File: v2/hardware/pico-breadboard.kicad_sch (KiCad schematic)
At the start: 39 parts, among them J1 Conn_01x05, J10 MPU6050 CONNECTOR, J11 Conn_01x03, J12 Conn_01x03, J2 LED, J3 5V CONNECTOR, J4 GND CONNECTOR, J5 3.3V CONNECTOR, J6 Conn_01x12, J7 Conn_01x11, J8 SCREEN CONNECTOR, J9 Conn_01x03, Q1 BC817, SW1 SW_SPST, SW2 SW_SPST, SW3 SW_SPST, SW4 SW_SPST, SW5 RotaryEncoder_Switch_MP, U1 Pico

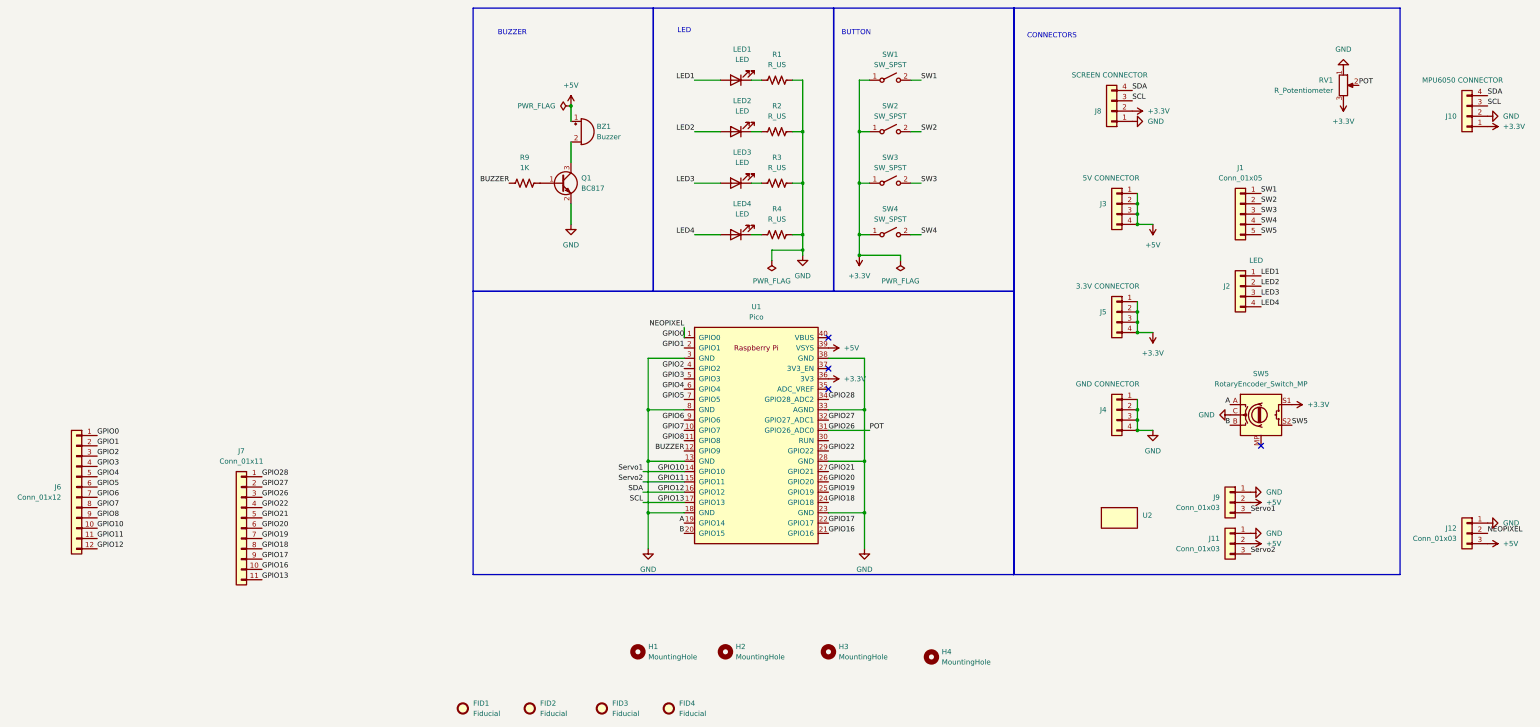
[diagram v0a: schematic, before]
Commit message: update
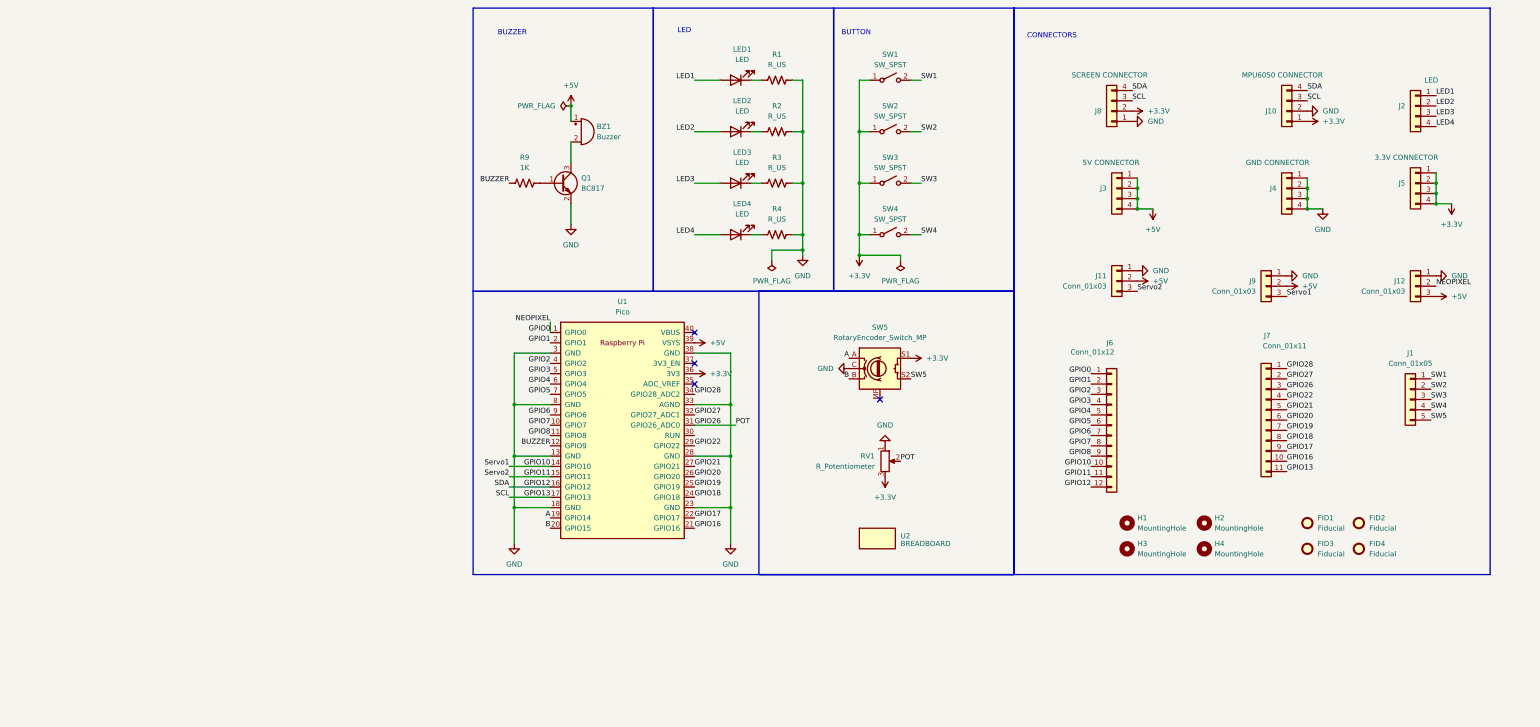
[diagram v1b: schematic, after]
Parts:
- U2: value ~ -> BREADBOARD
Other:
- moved on the sheet: FID1, FID2, FID3, FID4, H1, H2, H3, H4, J1, J10, J11, J12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

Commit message: update
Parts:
- FID1, FID2, FID3, FID4: footprint Fiducial:Fiducial_1mm_Mask2mm -> Library:Fiducial_1mm_Mask2mm; symbol Mechanical:Fiducial -> Library:Fiducial
- H1, H2, H3, H4: footprint MountingHole:MountingHole_3mm -> Library:MountingHole_3mm; symbol Mechanical:MountingHole -> Library:MountingHole
- J1: footprint Connector_PinHeader_2.54mm:PinHeader_1x05_P2.54mm_Vertical -> Library:PinHeader_1x05_P2.54mm_Vertical; symbol Connector_Generic:Conn_01x05 -> Library:Conn_01x05
- J10, J2, J3, J4, J5, J8: footprint Connector_PinHeader_2.54mm:PinHeader_1x04_P2.54mm_Vertical -> Library:PinHeader_1x04_P2.54mm_Vertical
- J11, J12, J9: footprint Connector_PinHeader_2.54mm:PinHeader_1x03_P2.54mm_Vertical -> Library:PinHeader_1x03_P2.54mm_Vertical; symbol Connector_Generic:Conn_01x03 -> Library:Conn_01x03
- J6: footprint Connector_PinHeader_2.54mm:PinHeader_1x12_P2.54mm_Vertical -> Library:PinHeader_1x12_P2.54mm_Vertical; symbol Connector_Generic:Conn_01x12 -> Library:Conn_01x12
- J7: footprint Connector_PinHeader_2.54mm:PinHeader_1x11_P2.54mm_Vertical -> Library:PinHeader_1x11_P2.54mm_Vertical; symbol Connector_Generic:Conn_01x11 -> Library:Conn_01x11
- LED1, LED2, LED3, LED4: footprint LED_SMD:LED_0603_1608Metric -> Library:LED_0603_1608Metric
- Q1: footprint Package_TO_SOT_SMD:SOT-23 -> Library:SOT-23
- R1, R2, R3, R4, R9: footprint Resistor_SMD:R_0402_1005Metric -> Library:R_0402_1005Metric
- U1: footprint RPi_Pico:RPi_Pico_SMD_TH -> Library:RPi_Pico_SMD_TH
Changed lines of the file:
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@@
 	)
 	(symbol
-		(lib_id "Mechanical:Fiducial")
+		(lib_id "Library:Fiducial")
 		(at 228.6 146.05 0)
 		(unit 1)
@@
 			)
 		)
-		(property "Footprint" "Fiducial:Fiducial_1mm_Mask2mm"
+		(property "Footprint" "Library:Fiducial_1mm_Mask2mm"
 			(at 228.6 146.05 0)
 			(effects
@@
 	)
 	(symbol
-		(lib_id "Connector_Generic:Conn_01x11")
+		(lib_id "Library:Conn_01x11")
 		(at 218.44 120.65 0)
 		(mirror y)
@@
 			)
 		)
-		(property "Footprint" "Connector_PinHeader_2.54mm:PinHeader_1x11_P2.54mm_Vertical"
+		(property "Footprint" "Library:PinHeader_1x11_P2.54mm_Vertical"
 			(at 218.44 120.65 0)
 			(effects
@@
 	)
 	(symbol
-		(lib_id "Mechanical:Fiducial")
+		(lib_id "Library:Fiducial")
 		(at 228.6 152.4 0)
 		(unit 1)
@@
 			)
 		)
-		(property "Footprint" "Fiducial:Fiducial_1mm_Mask2mm"
+		(property "Footprint" "Library:Fiducial_1mm_Mask2mm"
 			(at 228.6 152.4 0)
 			(effects
@@
 			)
 		)
-		(property "Footprint" "Connector_PinHeader_2.54mm:PinHeader_1x04_P2.54mm_Vertical"
+		(property "Footprint" "Library:PinHeader_1x04_P2.54mm_Vertical"
 			(at 255.27 43.18 0)
 			(effects
@@
 			)
 		)
-		(property "Footprint" "Connector_PinHeader_2.54mm:PinHeader_1x04_P2.54mm_Vertical"
+		(property "Footprint" "Library:PinHeader_1x04_P2.54mm_Vertical"
 			(at 223.52 63.5 0)
 			(effects
@@
 			)
 		)
-		(property "Footprint" "Connector_PinHeader_2.54mm:PinHeader_1x04_P2.54mm_Vertical"
+		(property "Footprint" "Library:PinHeader_1x04_P2.54mm_Vertical"
 			(at 180.34 44.45 0)
 			(effects
@@
 	)
 	(symbol
-		(lib_id "Mechanical:MountingHole")
+		(lib_id "Library:MountingHole")
 		(at 184.15 152.4 0)
 		(unit 1)
@@
 			)
 		)
-		(property "Footprint" "MountingHole:MountingHole_3mm"
+		(property "Footprint" "Library:MountingHole_3mm"
 			(at 184.15 152.4 0)
 			(effects
@@
 			)
 		)
-		(property "Footprint" "Connector_PinHeader_2.54mm:PinHeader_1x04_P2.54mm_Vertical"
+		(property "Footprint" "Library:PinHeader_1x04_P2.54mm_Vertical"
 			(at 181.61 63.5 0)
 			(effects
@@
 			)
 		)
-		(property "Footprint" "Connector_PinHeader_2.54mm:PinHeader_1x04_P2.54mm_Vertical"
+		(property "Footprint" "Library:PinHeader_1x04_P2.54mm_Vertical"
 			(at 223.52 44.45 0)
 			(effects
@@
 			)
 		)
-		(property "Footprint" "RPi_Pico:RPi_Pico_SMD_TH"
+		(property "Footprint" "Library:RPi_Pico_SMD_TH"
 			(at 59.69 123.19 90)
 			(effects
@@
 			)
 		)
-		(property "Footprint" "Resistor_SMD:R_0402_1005Metric"
+		(property "Footprint" "Library:R_0402_1005Metric"
 			(at 35.814 61.214 90)
 			(effects
@@
 	)
 	(symbol
-		(lib_id "Connector_Generic:Conn_01x03")
+		(lib_id "Library:Conn_01x03")
 		(at 181.61 86.36 0)
 		(mirror y)
@@
 			)
 		)
-		(property "Footprint" "Connector_PinHeader_2.54mm:PinHeader_1x03_P2.54mm_Vertical"
+		(property "Footprint" "Library:PinHeader_1x03_P2.54mm_Vertical"
 			(at 181.61 86.36 0)
 			(effects
@@
 			)
 		)
-		(property "Footprint" "LED_SMD:LED_0603_1608Metric"
+		(property "Footprint" "Library:LED_0603_1608Metric"
 			(at 87.63 62.23 0)
 			(effects
@@
 	)
 	(symbol
-		(lib_id "Mechanical:Fiducial")
+		(lib_id "Library:Fiducial")
 		(at 241.3 152.4 0)
 		(unit 1)
@@
 			)
 		)
-		(property "Footprint" "Fiducial:Fiducial_1mm_Mask2mm"
+		(property "Footprint" "Library:Fiducial_1mm_Mask2mm"
 			(at 241.3 152.4 0)
 			(effects
@@
 	)
 	(symbol
-		(lib_id "Connector_Generic:Conn_01x03")
+		(lib_id "Library:Conn_01x03")
 		(at 255.27 87.63 0)
 		(mirror y)
@@
 			)
 		)
-		(property "Footprint" "Connector_PinHeader_2.54mm:PinHeader_1x03_P2.54mm_Vertical"
+		(property "Footprint" "Library:PinHeader_1x03_P2.54mm_Vertical"
 			(at 255.27 87.63 0)
 			(effects
@@
 			)
 		)
-		(property "Footprint" "Resistor_SMD:R_0402_1005Metric"
+		(property "Footprint" "Library:R_0402_1005Metric"
 			(at 98.044 35.814 90)
 			(effects
@@
 	)
 	(symbol
-		(lib_id "Mechanical:MountingHole")
+		(lib_id "Library:MountingHole")
 		(at 203.2 152.4 0)
 		(unit 1)
@@
 			)
 		)
-		(property "Footprint" "MountingHole:MountingHole_3mm"
+		(property "Footprint" "Library:MountingHole_3mm"
 			(at 203.2 152.4 0)
 			(effects
@@
 	)
 	(symbol
-		(lib_id "Connector_Generic:Conn_01x05")
+		(lib_id "Library:Conn_01x05")
 		(at 254 115.57 0)
 		(mirror y)
@@
 			)
 		)
-		(property "Footprint" "Connector_PinHeader_2.54mm:PinHeader_1x05_P2.54mm_Vertical"
+		(property "Footprint" "Library:PinHeader_1x05_P2.54mm_Vertical"
 			(at 254 115.57 0)
 			(effects
@@
 			)
 		)
-		(property "Footprint" "Connector_PinHeader_2.54mm:PinHeader_1x04_P2.54mm_Vertical"
+		(property "Footprint" "Library:PinHeader_1x04_P2.54mm_Vertical"
 			(at 255.27 62.23 0)
 			(effects
@@
 			)
 		)
-		(property "Footprint" "Resistor_SMD:R_0402_1005Metric"
+		(property "Footprint" "Library:R_0402_1005Metric"
 			(at 98.044 61.214 90)
 			(effects
@@
 	)
 	(symbol
-		(lib_id "Connector_Generic:Conn_01x03")
+		(lib_id "Library:Conn_01x03")
 		(at 218.44 87.63 0)
 		(mirror y)
@@
 			)
 		)
-		(property "Footprint" "Connector_PinHeader_2.54mm:PinHeader_1x03_P2.54mm_Vertical"
+		(property "Footprint" "Library:PinHeader_1x03_P2.54mm_Vertical"
 			(at 218.44 87.63 0)
 			(effects
@@
 			)
 		)
-		(property "Footprint" "Resistor_SMD:R_0402_1005Metric"
+		(property "Footprint" "Library:R_0402_1005Metric"
 			(at 98.044 48.514 90)
 			(effects
@@
 	)
 	(symbol
-		(lib_id "Connector_Generic:Conn_01x12")
+		(lib_id "Library:Conn_01x12")
 		(at 180.34 121.92 0)
 		(unit 1)
@@
 			)
 		)
-		(property "Footprint" "Connector_PinHeader_2.54mm:PinHeader_1x12_P2.54mm_Vertical"
+		(property "Footprint" "Library:PinHeader_1x12_P2.54mm_Vertical"
 			(at 180.34 121.92 0)
 			(effects
@@
 	)
 	(symbol
-		(lib_id "Mechanical:MountingHole")
+		(lib_id "Library:MountingHole")
 		(at 184.15 146.05 0)
 		(unit 1)
@@
 			)
 		)
-		(property "Footprint" "MountingHole:MountingHole_3mm"
+		(property "Footprint" "Library:MountingHole_3mm"
 			(at 184.15 146.05 0)
 			(effects
@@
 	)
 	(symbol
-		(lib_id "Mechanical:MountingHole")
+		(lib_id "Library:MountingHole")
 		(at 203.2 146.05 0)
 		(unit 1)
@@
 			)
 		)
-		(property "Footprint" "MountingHole:MountingHole_3mm"
+		(property "Footprint" "Library:MountingHole_3mm"
 			(at 203.2 146.05 0)
 			(effects
@@
 	)
 	(symbol
-		(lib_id "Mechanical:Fiducial")
+		(lib_id "Library:Fiducial")
 		(at 241.3 146.05 0)
 		(unit 1)
@@
 			)
 		)
-		(property "Footprint" "Fiducial:Fiducial_1mm_Mask2mm"
+		(property "Footprint" "Library:Fiducial_1mm_Mask2mm"
 			(at 241.3 146.05 0)
 			(effects
@@
 			)
 		)
-		(property "Footprint" "LED_SMD:LED_0603_1608Metric"
+		(property "Footprint" "Library:LED_0603_1608Metric"
 			(at 87.63 74.93 0)
 			(effects
@@
 			)
 		)
-		(property "Footprint" "Resistor_SMD:R_0402_1005Metric"
+		(property "Footprint" "Library:R_0402_1005Metric"
 			(at 98.044 73.914 90)
 			(effects
@@
 			)
 		)
-		(property "Footprint" "LED_SMD:LED_0603_1608Metric"
+		(property "Footprint" "Library:LED_0603_1608Metric"
 			(at 87.63 49.53 0)
 			(effects
@@
 			)
 		)
-		(property "Footprint" "Package_TO_SOT_SMD:SOT-23"
+		(property "Footprint" "Library:SOT-23"
 			(at 49.53 64.135 0)
 			(effects
@@
 			)
 		)
-		(property "Footprint" "LED_SMD:LED_0603_1608Metric"
+		(property "Footprint" "Library:LED_0603_1608Metric"
 			(at 87.63 36.83 0)
 			(effects
